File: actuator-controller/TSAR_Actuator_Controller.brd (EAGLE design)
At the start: 147.6 x 77.7 mm, 168 parts, among them Q1 220mA/50V/3.5Ω, Q10 220mA/50V/3.5Ω, Q11 IRF9530, Q12 220mA/50V/3.5Ω, Q13 IRF9530, Q14 220mA/50V/3.5Ω, Q15 IRF9530, Q16 220mA/50V/3.5Ω, Q17 IRF9530, Q18 220mA/50V/3.5Ω, Q19 IRF9530, Q2 IRF9530, Q20 220mA/50V/3.5Ω, Q3 IRF9530, Q4 220mA/50V/3.5Ω, Q5 IRF9530, Q6 220mA/50V/3.5Ω, Q7 IRF9530, Q8 220mA/50V/3.5Ω, Q9 IRF9530

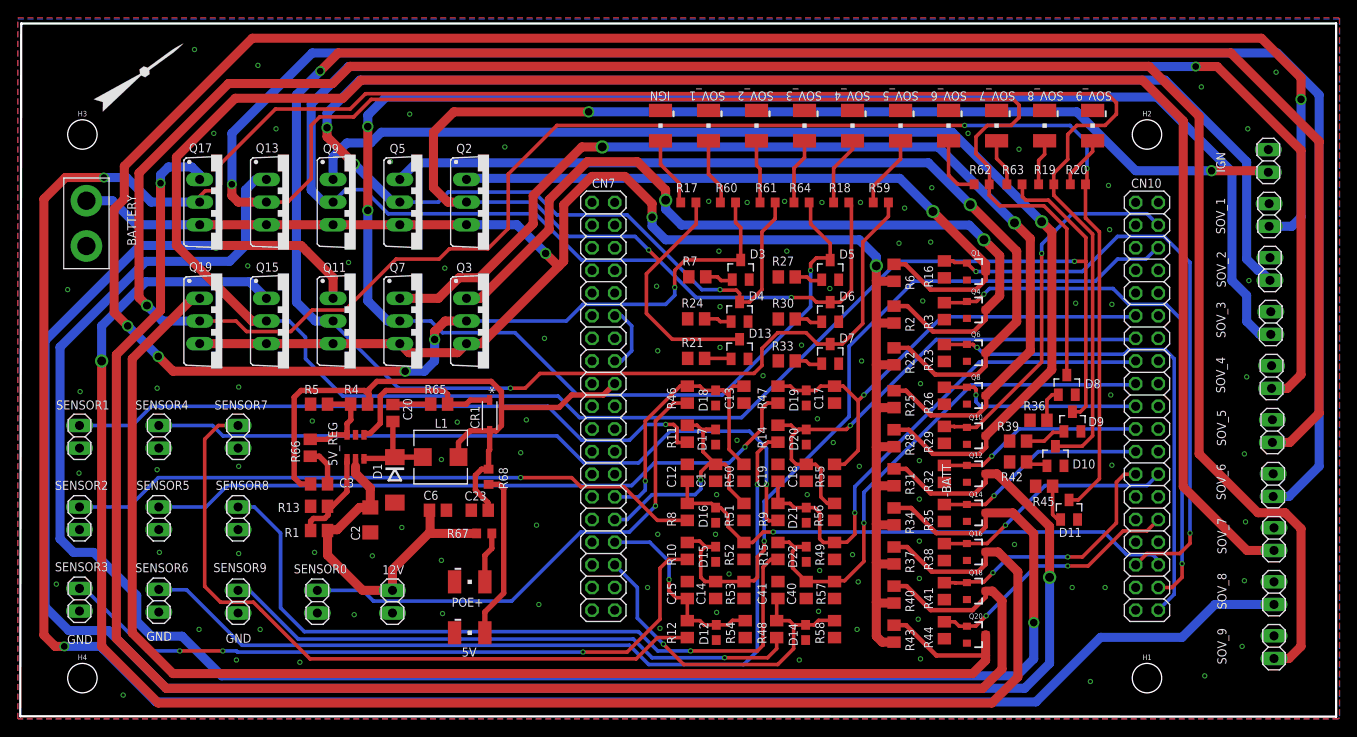
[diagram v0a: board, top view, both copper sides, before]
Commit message: thick routes on AC board. protections on SFE
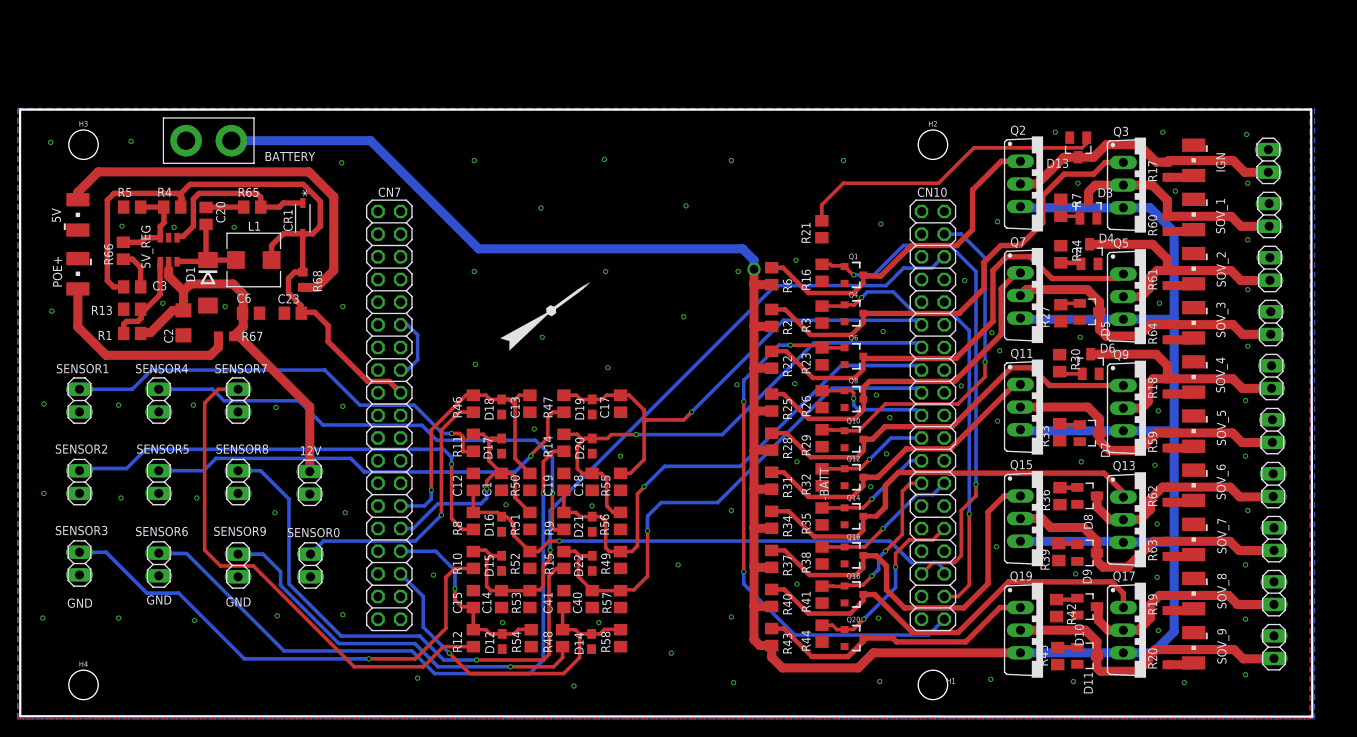
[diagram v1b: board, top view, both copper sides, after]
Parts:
- moved Q17 114.2 mm to (126.3, 9.18)
- moved Q13 102.5 mm to (126.3, 21.6)
- moved Q19 98.3 mm to (114.7, 9.18)
- moved Q9 91.6 mm to (126.3, 34.1)
- moved Q15 87.4 mm to (114.7, 21.7)
- moved Q5 81.8 mm to (126.3, 46.6)
- moved Q11 77.7 mm to (114.7, 34.2)
- moved Q3 75.2 mm to (126.3, 59.1)
- moved Q7 69.7 mm to (114.7, 46.7)
- moved 5V 64.2 mm to (6.48, 55.8), turned to 0 degrees
- moved Q2 62.2 mm to (114.7, 59.2)
- moved IGN. 59.9 mm to (131.6, 61.9)
- moved SOV_9. 59.6 mm to (131.6, 7.21)
- moved POE+ 55.9 mm to (6.48, 49.1), turned to 180 degrees
- moved SOV_1. 55.3 mm to (131.6, 55.8)
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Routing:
- net SOL_GPIO_18: track 372.7 -> 24.7 mm, vias 2 -> 0
- net SOL_GPIO_19: track 374.3 -> 33.8 mm, vias 3 -> 0
- net SOL_GPIO_17: track 332.2 -> 33.7 mm, vias 1 -> 0
- net SOL_GPIO_16: track 320.9 -> 24.3 mm, vias 1 -> 0
- net SOL_GPIO_11: track 264.6 -> 24.3 mm, vias 6 -> 0
- net SOL_GPIO_15: track 268.6 -> 32.9 mm, vias 2 -> 0
- net SOL_GPIO_14: track 232.9 -> 30.2 mm, vias 2 -> 0
- net N$39: track 225.9 -> 34.8 mm, vias 2 -> 0
- net SOL_GPIO_13: track 215.8 -> 33.3 mm, vias 3 -> 0
- net SOL_GPIO_12: track 194.5 -> 29.5 mm, vias 3 -> 0
- net N$41: track 207.8 -> 47.4 mm, vias 1 -> 0
- net N$43: track 193.3 -> 44.7 mm, vias 1 -> 0
- net N$45: track 184.8 -> 48.1 mm, vias 1 -> 0
- net SOL_GPIO_10: track 158.7 -> 31.1 mm, vias 3 -> 0
- net N$47: track 153.9 -> 32.0 mm
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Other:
- board size 147.6 x 77.7 mm -> 144.9 x 68.1 mm
- board text removed: "IGN"
- board text removed: "SOV_1"
- board text removed: "SOV_2"
- board text removed: "SOV_3"
- board text removed: "SOV_4"
- board text removed: "SOV_5"
- board text removed: "SOV_6"
- board text removed: "SOV_7"
- board text removed: "SOV_8"
- board text removed: "SOV_9"

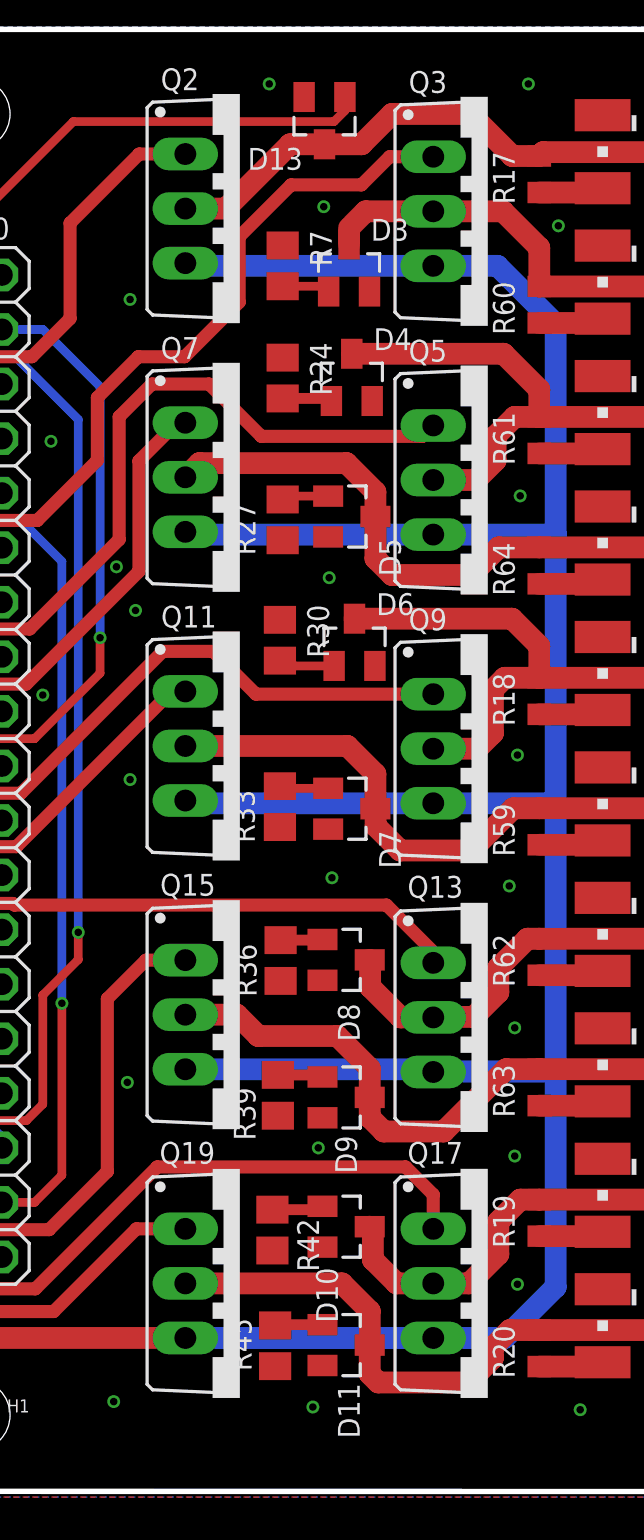
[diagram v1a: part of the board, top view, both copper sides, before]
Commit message: label correction
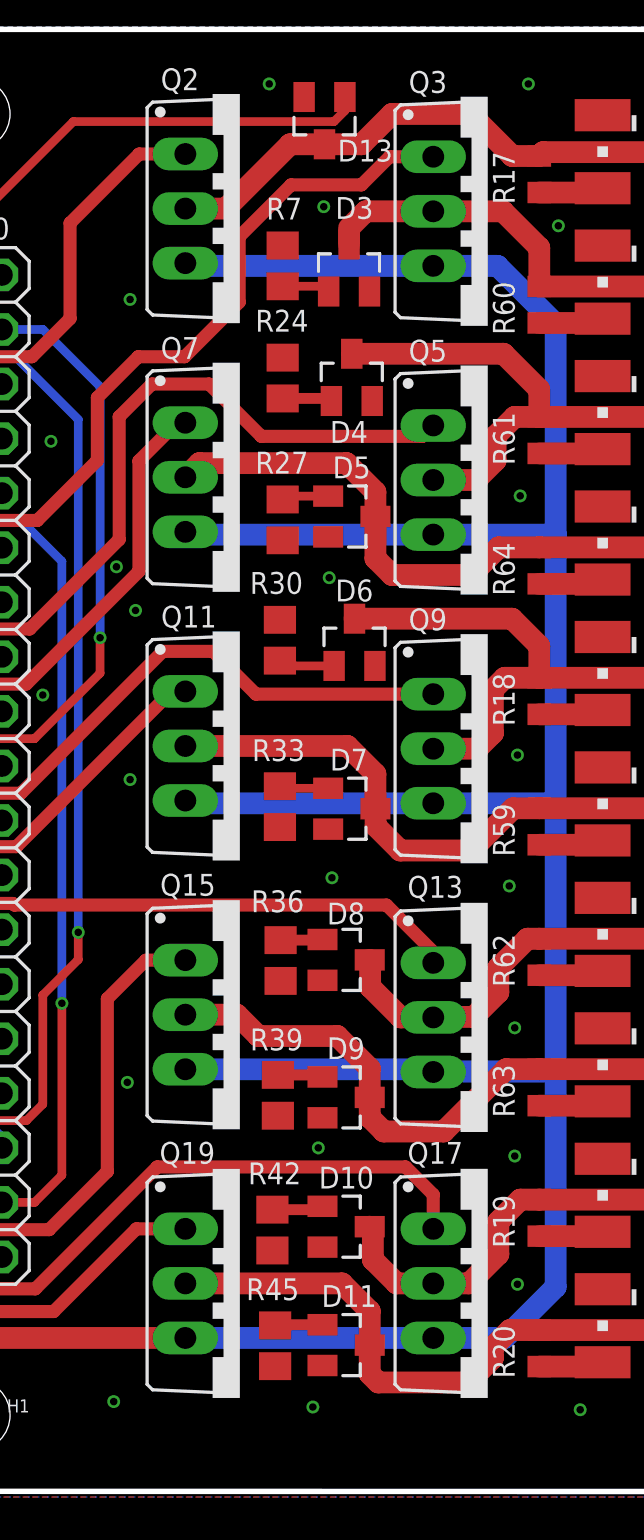
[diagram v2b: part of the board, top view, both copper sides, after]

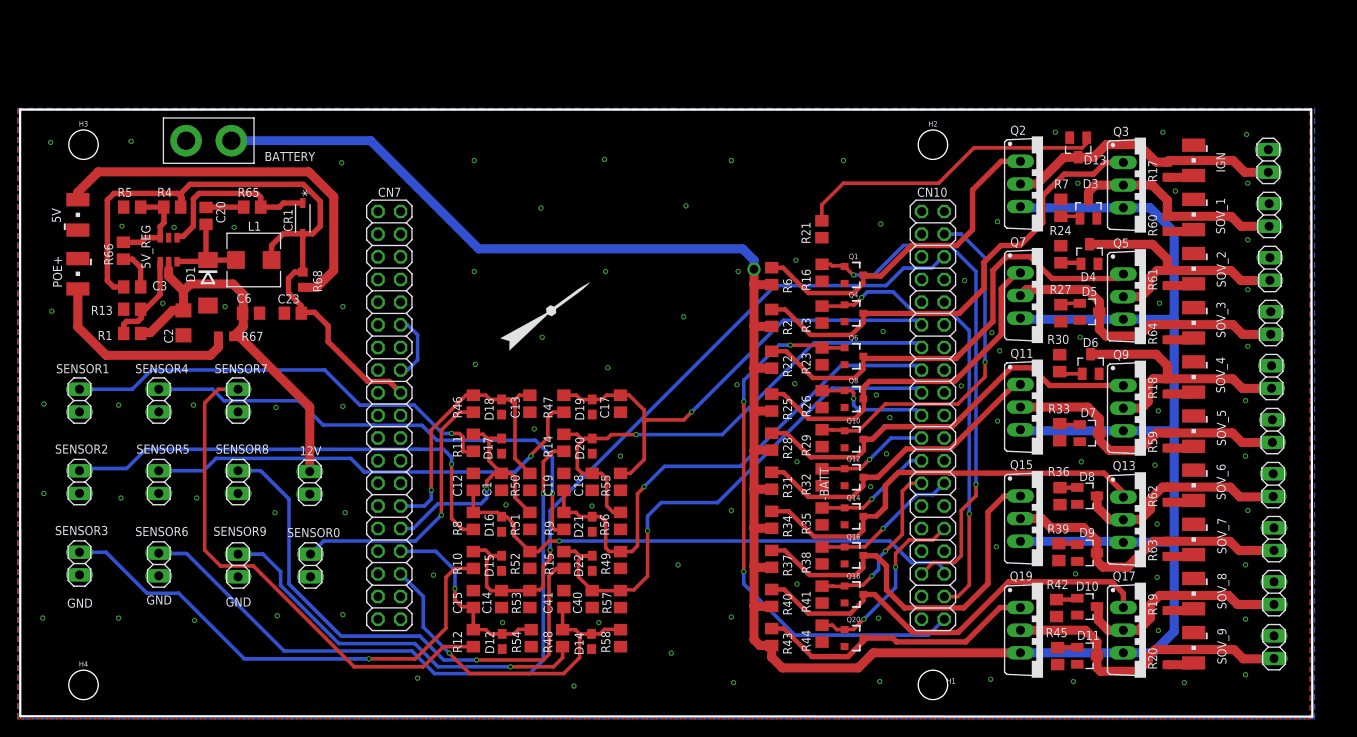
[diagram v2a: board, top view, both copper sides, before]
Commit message: Minor cleanup around the SPS, minor polish on ground and on vbatt distribution.
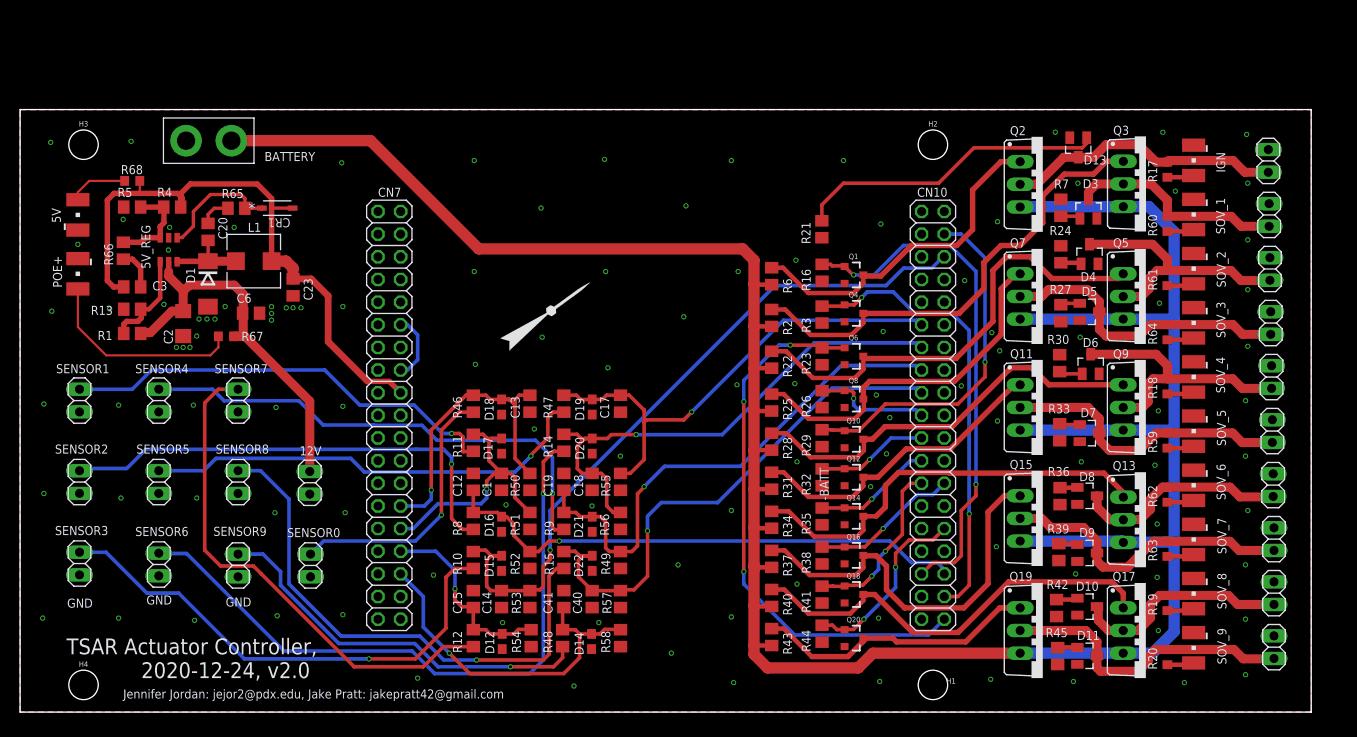
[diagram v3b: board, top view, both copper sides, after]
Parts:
- moved R68 22.1 mm to (12.6, 59.6), turned to 0 degrees
- moved CR1 3.09 mm to (28.8, 56.5), turned to 0 degrees
- moved C23 2.89 mm to (30.6, 47.6), turned to 270 degrees
- moved C20 1.81 mm to (21.1, 53.8)
- moved R65 1.78 mm to (24.3, 56.5)
- moved D1 0.13 mm to (21.1, 48.0)
- moved L1 0.13 mm to (26.2, 50.6)
- moved Q3 0.13 mm to (126.3, 59.2)
- moved Q7 0.11 mm to (114.7, 46.6)
- moved C2 0.09 mm to (18.3, 43.6)
- moved Q9 0.09 mm to (126.2, 34.2)
- moved Q11 0.05 mm to (114.7, 34.2)
- moved Q19 0.05 mm to (114.7, 9.14)
- moved Q2 0.05 mm to (114.7, 59.2)
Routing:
- net N$35: track 44.2 -> 6.61 mm
- net +5V: track 77.0 -> 69.1 mm
- net N$4: track 19.4 -> 13.8 mm
- net VBATT: track 290.9 -> 293.2 mm, vias 1 -> 0
- net N$8: track 10.8 -> 8.97 mm
- net +12V: track 43.8 -> 44.8 mm
- net N$26: track 4.25 -> 3.53 mm
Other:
- board size 144.9 x 68.1 mm -> 144.8 x 67.6 mm
- board text added: "TSAR Actuator Controller, 2020-12-24, v2.0"
- board text removed: "TSAR Actuator Controller, 2020 Dec 24, Version: 2.0"
